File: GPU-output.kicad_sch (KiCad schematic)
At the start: 26 parts, among them J1 Conn_1-2212115-4, Q1 BSS138PW, Q2 SI7613DN-T1-GE3, Q3 SI7613DN-T1-GE3, U33 SN74LV1T125DBVR, U4 TMCS1100A2-Q1

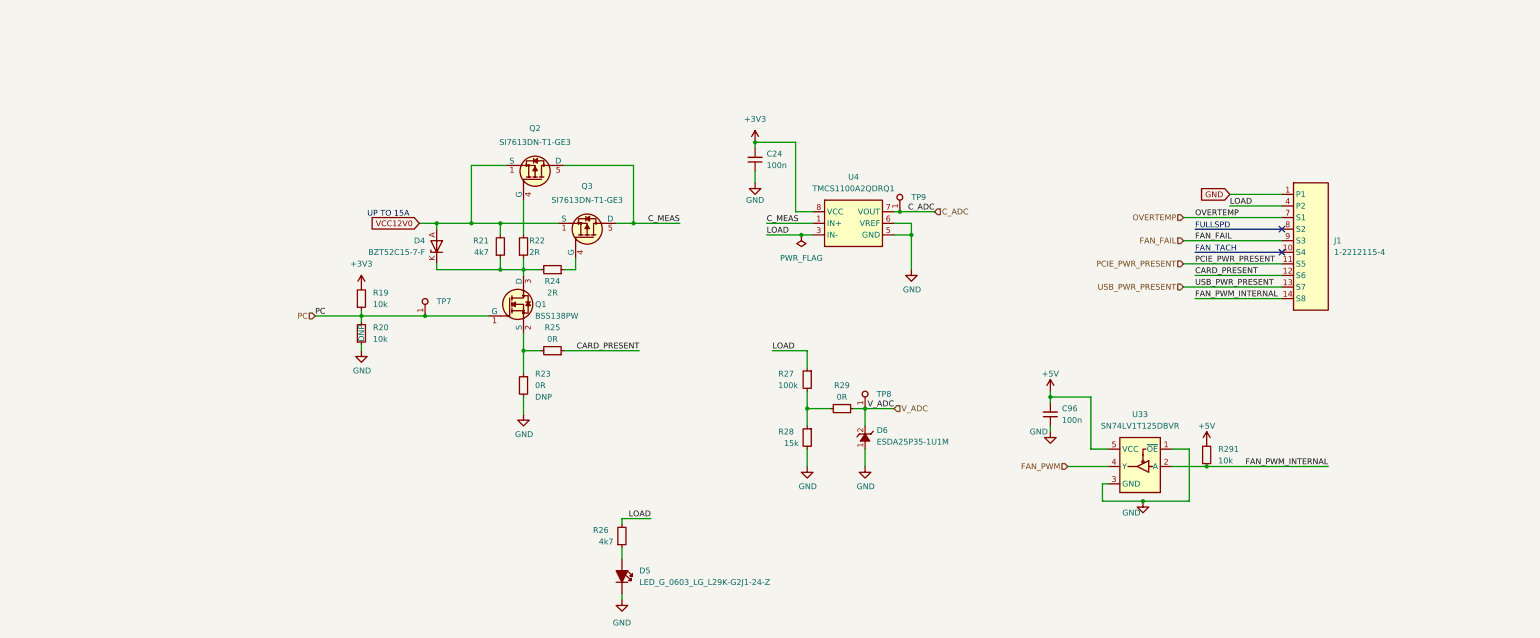
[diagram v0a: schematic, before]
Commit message: Cleanup schematic
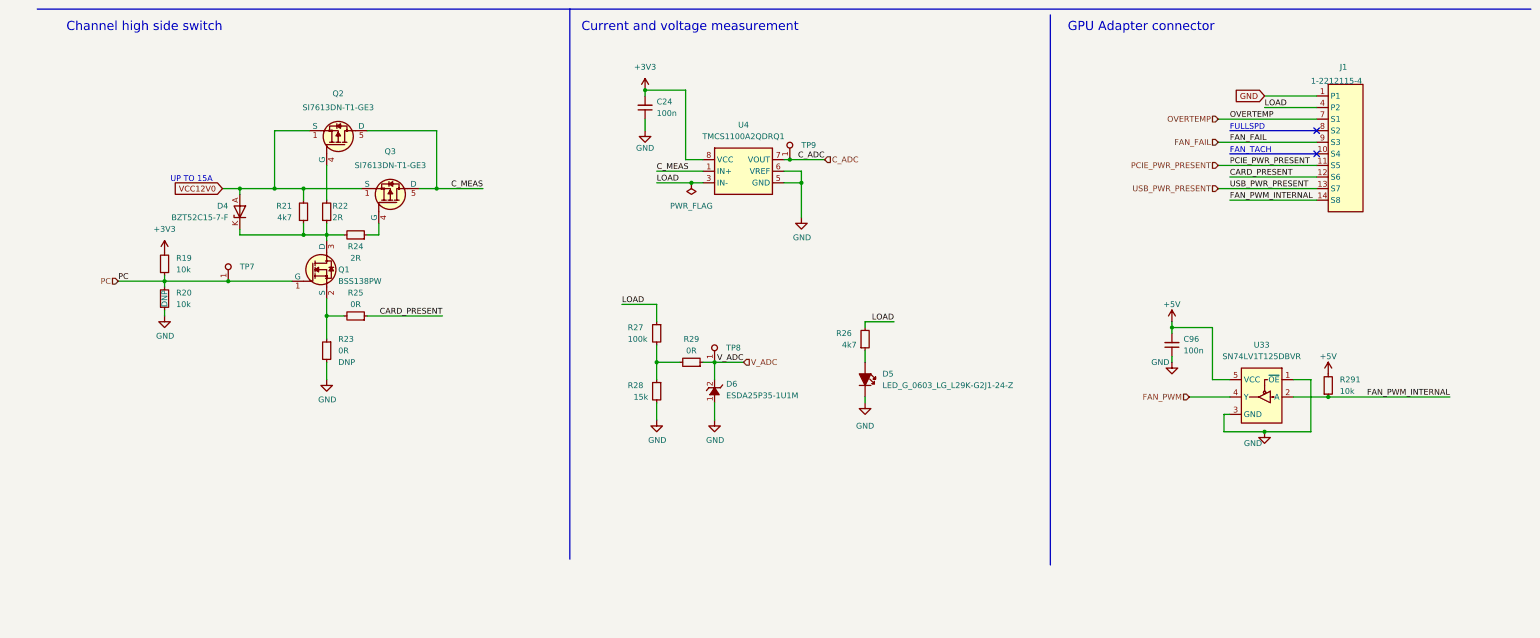
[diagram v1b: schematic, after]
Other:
- note added: "Channel high side switch"
- note added: "Current and voltage measurement"
- note added: "GPU Adapter connector"
- moved on the sheet: C24, C96, D4, D5, D6, J1, Q1, Q2, Q3, R19, R20, R21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
